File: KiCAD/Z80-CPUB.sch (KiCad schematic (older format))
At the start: 29 parts, among them J1 SBC8080 BUS, J2 Jack-DC, M1 MountingHole_3M, M2 MountingHole_3M, M3 MountingHole_3M, M4 MountingHole_3M, SW1 RESET SW, U1 Z80CPU, U2 74HC14, U3 74HC04, U4 74HC32, Y1 7.3728MHz

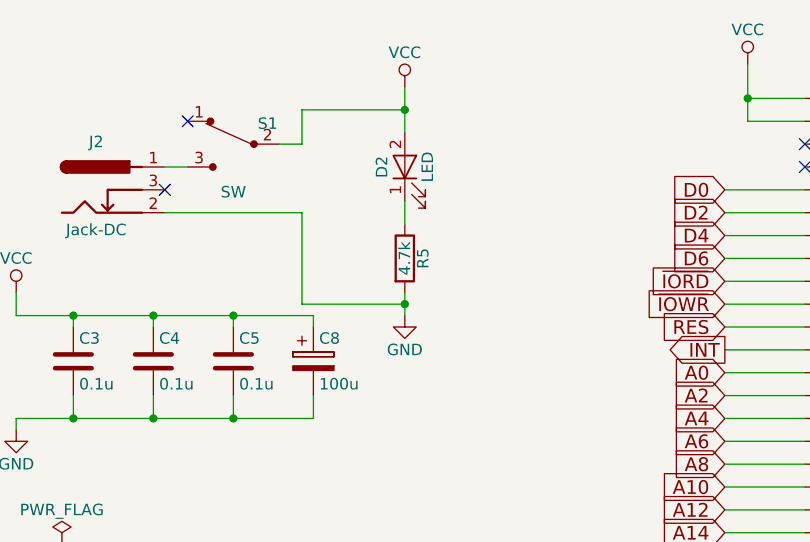
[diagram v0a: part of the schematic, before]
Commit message: r1.1 最終確認
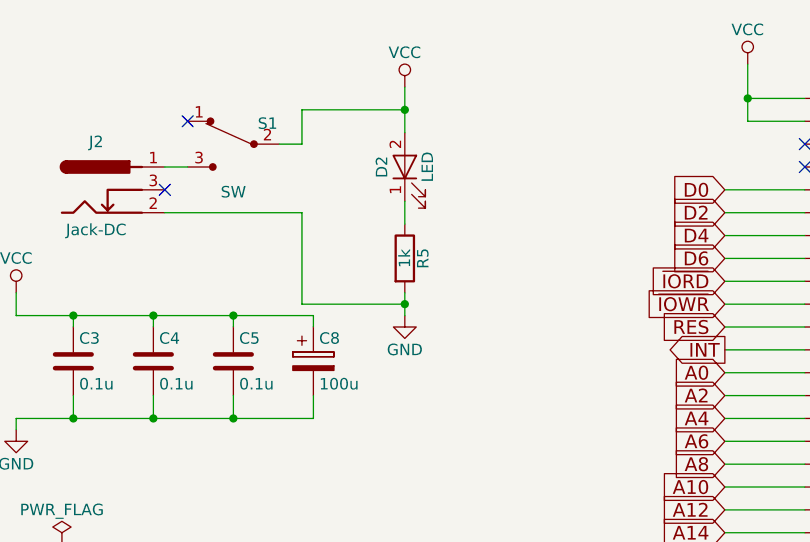
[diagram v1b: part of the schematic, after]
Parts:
- R5: value 4.7k -> 1k
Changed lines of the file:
@@
 P 7750 1650
 F 0 "R5" V 7830 1650 50  0000 C CNN
-F 1 "4.7k" V 7750 1650 50  0000 C CNN
+F 1 "1k" V 7750 1650 50  0000 C CNN
 F 2 "Resistors_THT:R_Axial_DIN0207_L6.3mm_D2.5mm_P7.62mm_Horizontal" V 7680 1650 50  0001 C CNN
 F 3 "" H 7750 1650 50  0001 C CNN

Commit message: REV2 回路図、製造データ出力
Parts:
- added C10, C9: 0.1u, Capacitor_THT:C_Disc_D3.0mm_W2.0mm_P2.50mm, symbol Device:C
- added R6, R7: 4.7k, Resistor_THT:R_Axial_DIN0207_L6.3mm_D2.5mm_P10.16mm_Horizontal, symbol Device:R
- added U5: 74HC32, Package_DIP:DIP-14_W7.62mm_Socket, symbol 74xx:74LS32
- added U6: 74HC125, Package_DIP:DIP-14_W7.62mm_Socket, symbol 74xx:74LS125
- C1, C3, C4, C5, C6, C7: footprint Capacitors_THT:C_Rect_L4.0mm_W2.5mm_P2.50mm -> Capacitor_THT:C_Disc_D3.0mm_W2.0mm_P2.50mm
- D1: footprint Diodes_THT:D_DO-41_SOD81_P10.16mm_Horizontal -> Diode_THT:D_A-405_P10.16mm_Horizontal
- D2: footprint LEDs:LED_D3.0mm -> LED_THT:LED_D3.0mm
- J1: footprint Pin_Headers:Pin_Header_Angled_2x20 -> Connector_PinHeader_2.54mm:PinHeader_2x20_P2.54mm_Horizontal
- M1, M2, M3, M4: footprint Mounting_Holes:MountingHole_3.2mm_M3 -> MountingHole:MountingHole_3.2mm_M3
- R1: value 3.3k -> 4.7k; footprint Resistors_THT:R_Axial_DIN0207_L6.3mm_D2.5mm_P7.62mm_Horizontal -> Resistor_THT:R_Axial_DIN0207_L6.3mm_D2.5mm_P10.16mm_Horizontal
- R2: value 2.2k -> 4.7k; footprint Resistors_THT:R_Axial_DIN0207_L6.3mm_D2.5mm_P7.62mm_Horizontal -> Resistor_THT:R_Axial_DIN0207_L6.3mm_D2.5mm_P10.16mm_Horizontal
- R3, R4, R5: footprint Resistors_THT:R_Axial_DIN0207_L6.3mm_D2.5mm_P7.62mm_Horizontal -> Resistor_THT:R_Axial_DIN0207_L6.3mm_D2.5mm_P10.16mm_Horizontal
- RN1: value R_Network08 -> 10k
- S1: footprint digikey-footprints:Switch_Slide_11.6x4mm_EG1218 -> Connector_PinSocket_2.54mm:PinSocket_1x03_P2.54mm_Vertical
- SW1: footprint Buttons_Switches_THT:SW_PUSH_6mm -> Button_Switch_THT:SW_PUSH_6mm_H4.3mm
- U1: footprint Housings_DIP:DIP-40_W15.24mm -> Package_DIP:DIP-40_W15.24mm_Socket
- U2, U3, U4: footprint Housings_DIP:DIP-14_W7.62mm_Socket -> Package_DIP:DIP-14_W7.62mm_Socket
- Y1: footprint Crystals:Crystal_HC49-4H_Vertical -> Crystal:Crystal_HC49-U_Vertical
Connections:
- net labels added: HLDA, HOLD, RDYIN, ~INTA, ~RESIN
- wire segments 207 -> 275
- no-connect marks 18 -> 12
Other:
- moved on the sheet: C1, C2, C3, C4, C5, C6, C7, C8, D1, D2, J1, J2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

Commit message: REV2.1検討開始 回路図、パターン変更
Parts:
- added C11, C12: 0.1u, Capacitor_THT:C_Disc_D3.0mm_W2.0mm_P2.50mm, symbol Device:C
- added U7: 74HC74, Package_DIP:DIP-14_W7.62mm_Socket, symbol 74xx:74HC74
- added U8: 74LS08, Package_DIP:DIP-14_W7.62mm_Socket, symbol 74xx:74LS08
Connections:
- net labels added: ~RESET
- wire segments 275 -> 332
- no-connect marks 12 -> 14
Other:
- moved on the sheet: C10, C3, C4, C5, C8, C9, M1, M2, M3, M4, U5B, U5C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

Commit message: REV3基板パターン、ガーバーデータ出力
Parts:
- removed R6: 4.7k, Resistor_THT:R_Axial_DIN0207_L6.3mm_D2.5mm_P10.16mm_Horizontal, symbol Device:R
- added J3: Z80 CTL, Connector_PinHeader_2.54mm:PinHeader_2x07_P2.54mm_Horizontal, symbol Connector_Generic:Conn_02x07_Odd_Even
- added RN2: 4.7k, Resistor_THT:R_Array_SIP9, symbol Device:R_Network08
- RN1: footprint Resistors_THT:R_Array_SIP9 -> Resistor_THT:R_Array_SIP9
- U8: value 74LS08 -> 74HC08
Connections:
- net labels added: RN21, RN22, RN23, RN24, ~BUSACK, ~BUSREQ, ~BUSRQ-J, ~HALT, ~INT-J, ~M1, ~NMI, ~RFSH, ~WAIT
- wire segments 332 -> 366
- no-connect marks 14 -> 15
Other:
- moved on the sheet: C1, C10, C11, C12, C2, C3, C4, C5, C6, C7, C8, C9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
